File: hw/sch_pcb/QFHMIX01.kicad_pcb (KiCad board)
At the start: 2 copper layers, 90.9 x 90.9 mm, 205 parts, among them J1 HEADER_1x08, J2 +9V, M1 HOLE, M2 HOLE, M3 HOLE, M4 HOLE, M5 HOLE, M6 HOLE, M7 HOLE, M8 HOLE, U1 LM1117MP-3,3/NO, U11 TPS563249, U12 Si53322, U2 AD8343, U3 AD8343, U5 LT6604-10, U6 MPGA-105+, U7 MPGA-105+, U8 MGVA-63+, U9 MGVA-63+

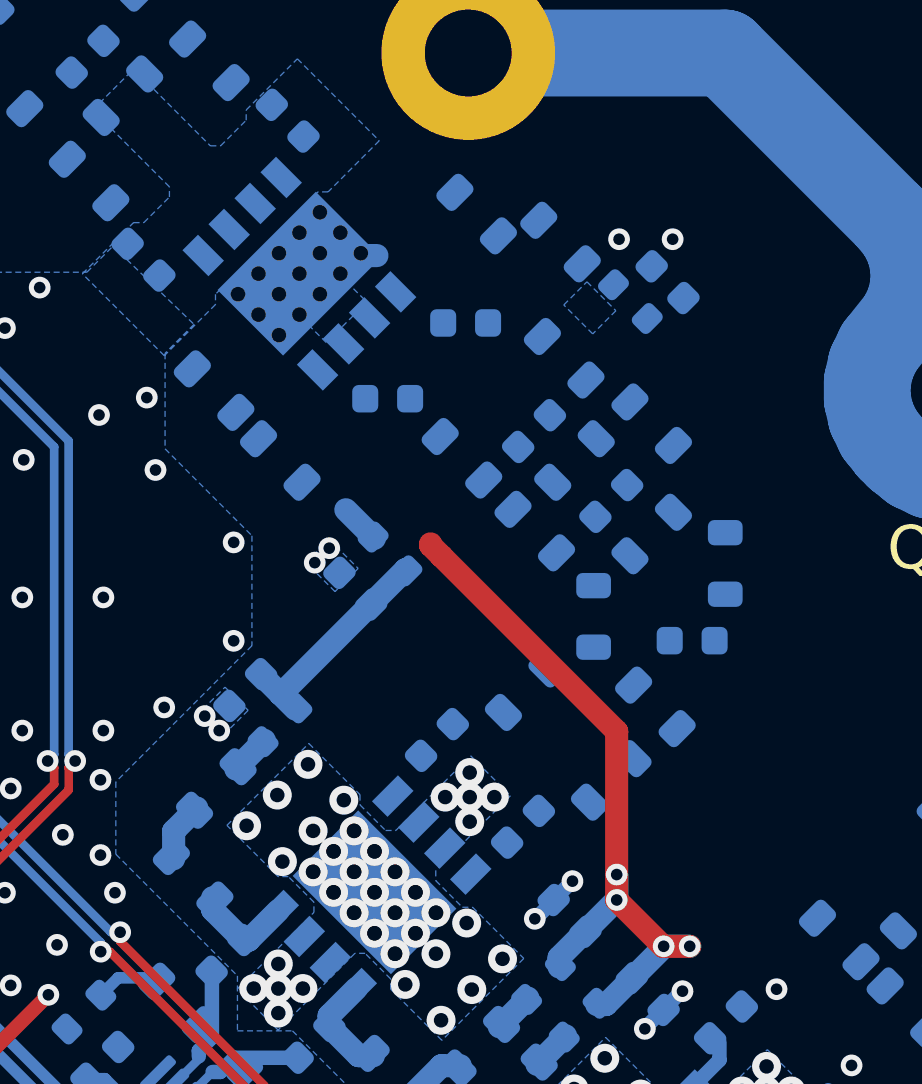
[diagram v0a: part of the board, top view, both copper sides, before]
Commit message: RF layout.
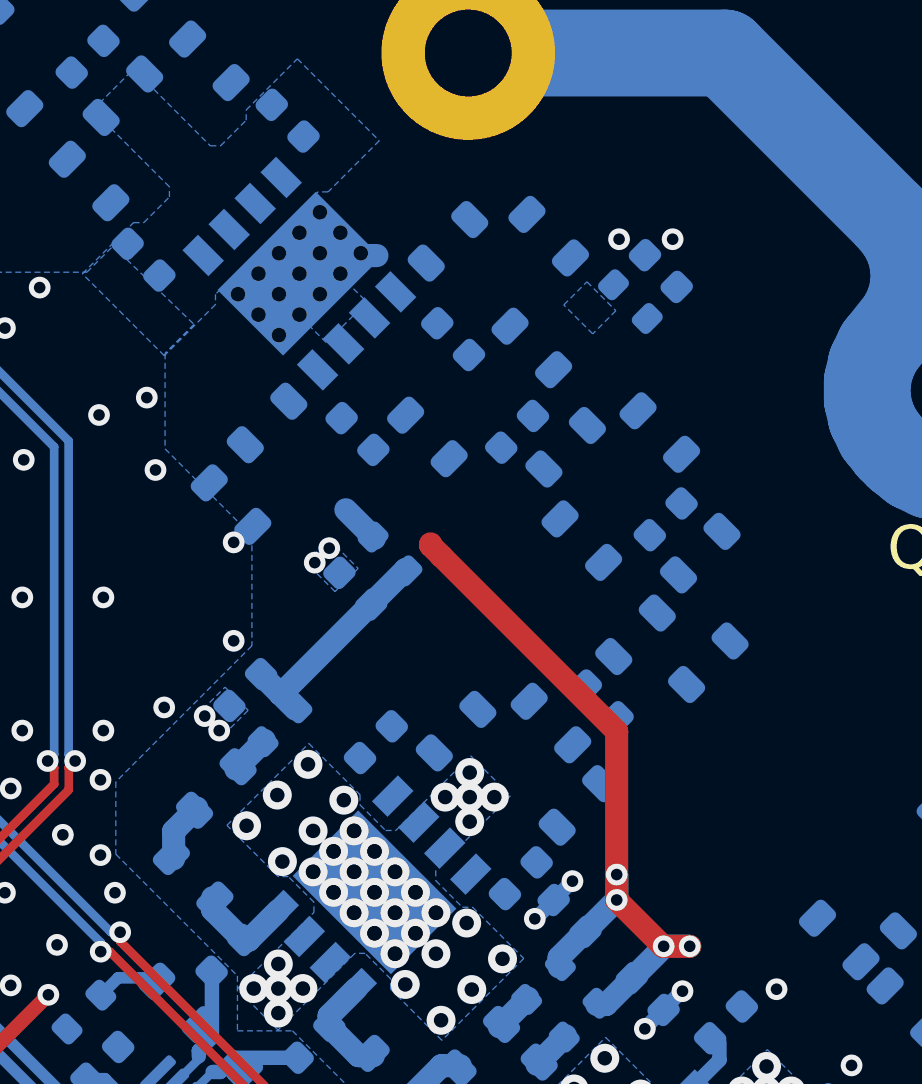
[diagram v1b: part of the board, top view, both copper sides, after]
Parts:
- moved C65 3.76 mm to (154.6, 76.4), turned to 135 degrees
- moved L67 3.65 mm to (152.9, 77.1)
- moved L65 3.48 mm to (158.3, 75.1), turned to 45 degrees
- moved L69 2.77 mm to (149.6, 77.4)
- moved L18 2.28 mm to (141.8, 69.6)
- moved L19 2.14 mm to (143.1, 66.8), turned to 45 degrees
- moved C29 2.11 mm to (146.8, 77.8)
- moved C63 1.98 mm to (156.8, 70.1)
- moved L36 1.80 mm to (158.0, 71.3)
- moved C30 1.78 mm to (151.8, 82.5)
- moved L60 1.66 mm to (153.9, 70.8)
- moved C49 1.60 mm to (146.2, 67.2), turned to 135 degrees
- moved L39 1.58 mm to (155.8, 74.1), turned to -135 degrees
- moved L63 1.41 mm to (153.8, 80.0)
- moved L58 1.40 mm to (148.6, 67.3)
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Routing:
- net Net-(L18-Pad1): vias 0 -> 1
- net GND: vias 290 -> 289
